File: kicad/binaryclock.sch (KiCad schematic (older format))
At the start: 10 parts, among them IC1 ATMEGA328P-PU, SW1 Reset, Y1 16MHz

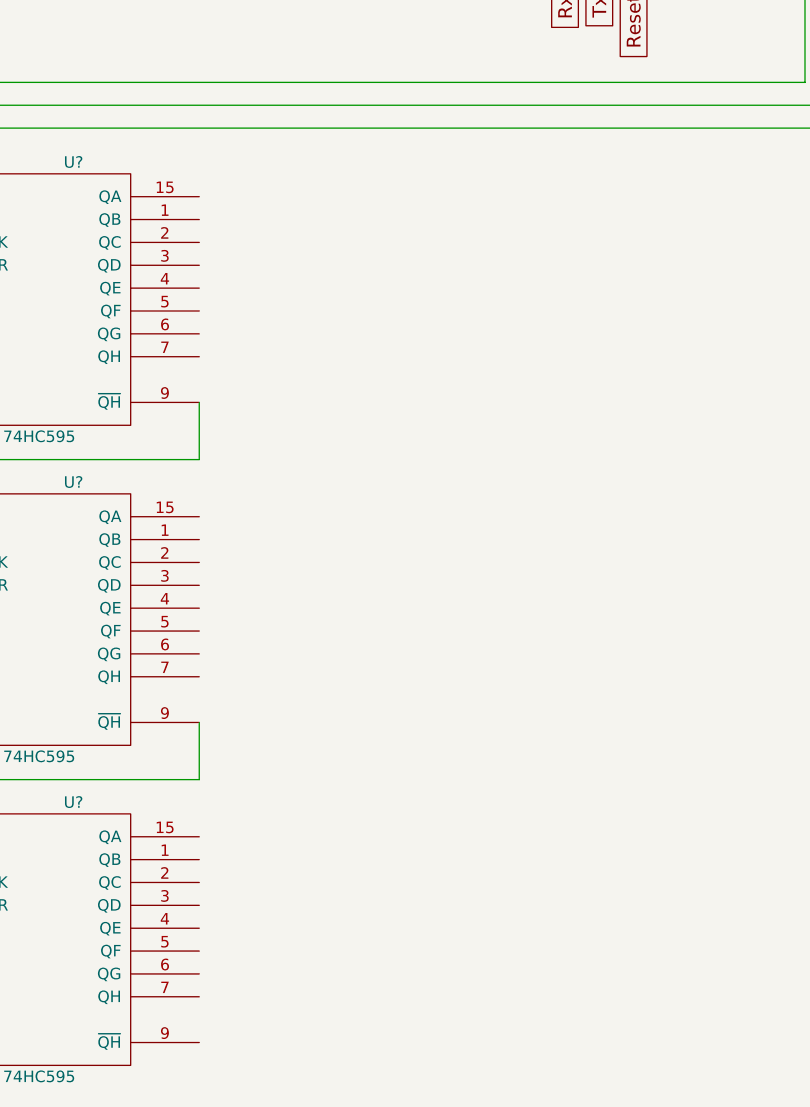
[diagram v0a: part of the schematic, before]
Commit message: update kicad
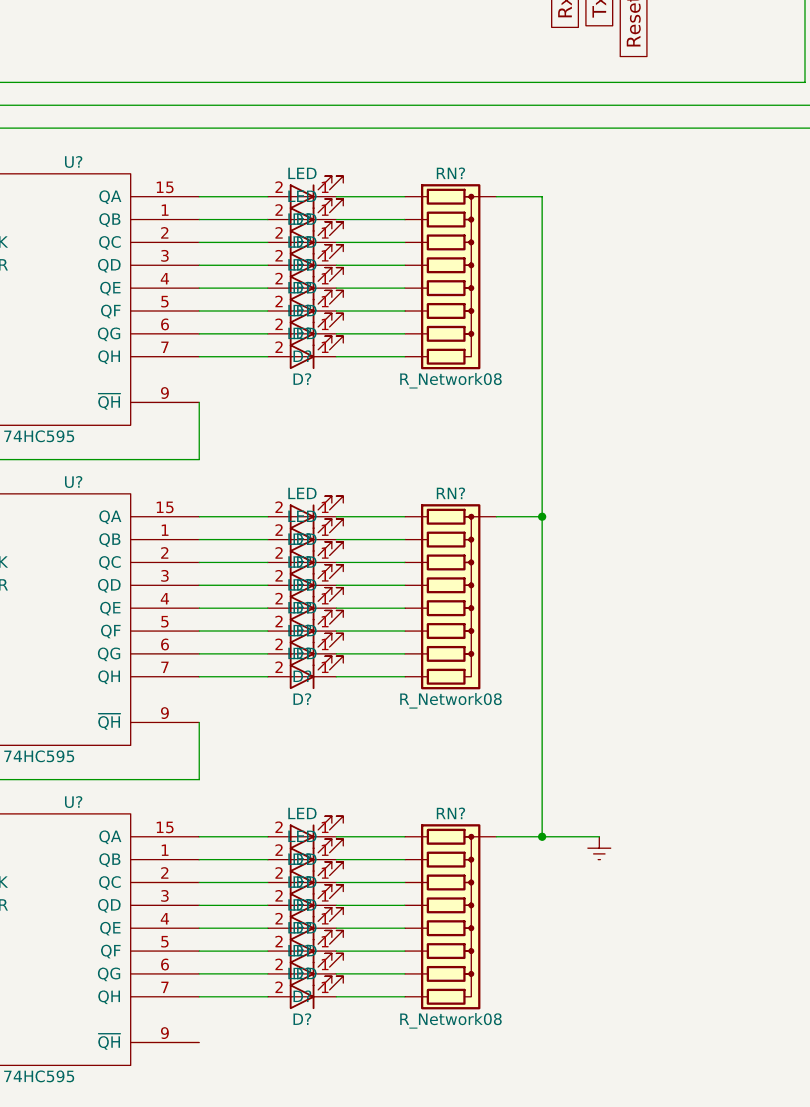
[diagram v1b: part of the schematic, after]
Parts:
- added D? (x24): LED, symbol LED
- added RN? (x3): R_Network08, Resistors_THT:R_Array_SIP9, symbol R_Network08
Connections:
- net Earth: now also RN?.1 (common), RN?.1 (common), RN?.1 (common)
- net at U?.1 (QB): now also D?.2 (A) (x3)
- net at U?.15 (QA): now also D?.2 (A) (x3)
- net at U?.2 (QC): now also D?.2 (A) (x3)
- net at U?.3 (QD): now also D?.2 (A) (x3)
- net at U?.4 (QE): now also D?.2 (A) (x3)
- net at U?.5 (QF): now also D?.2 (A) (x3)
- net at U?.6 (QG): now also D?.2 (A) (x3)
- net at U?.7 (QH): now also D?.2 (A) (x3)
- new net: D?.1 (K), RN?.2 (R1) (x3)
- new net: D?.1 (K), RN?.3 (R2) (x3)
- new net: D?.1 (K), RN?.4 (R3) (x3)
- new net: D?.1 (K), RN?.5 (R4) (x3)
- new net: D?.1 (K), RN?.6 (R5) (x3)
- new net: D?.1 (K), RN?.7 (R6) (x3)
- new net: D?.1 (K), RN?.8 (R7) (x3)
- new net: D?.1 (K), RN?.9 (R8) (x3)
